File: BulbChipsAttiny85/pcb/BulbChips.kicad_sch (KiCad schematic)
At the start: 27 parts, among them J1 USB_C_Receptacle_USB2.0_14P, J2 LED_2pin_Socket, SW1 SW_Push, U1 DMN52D0UV, U2 USBLC6-2P6, U3 S-82A1ACA-I6T1U, U4 ATtiny85-20M, U5 BQ24045DSQR

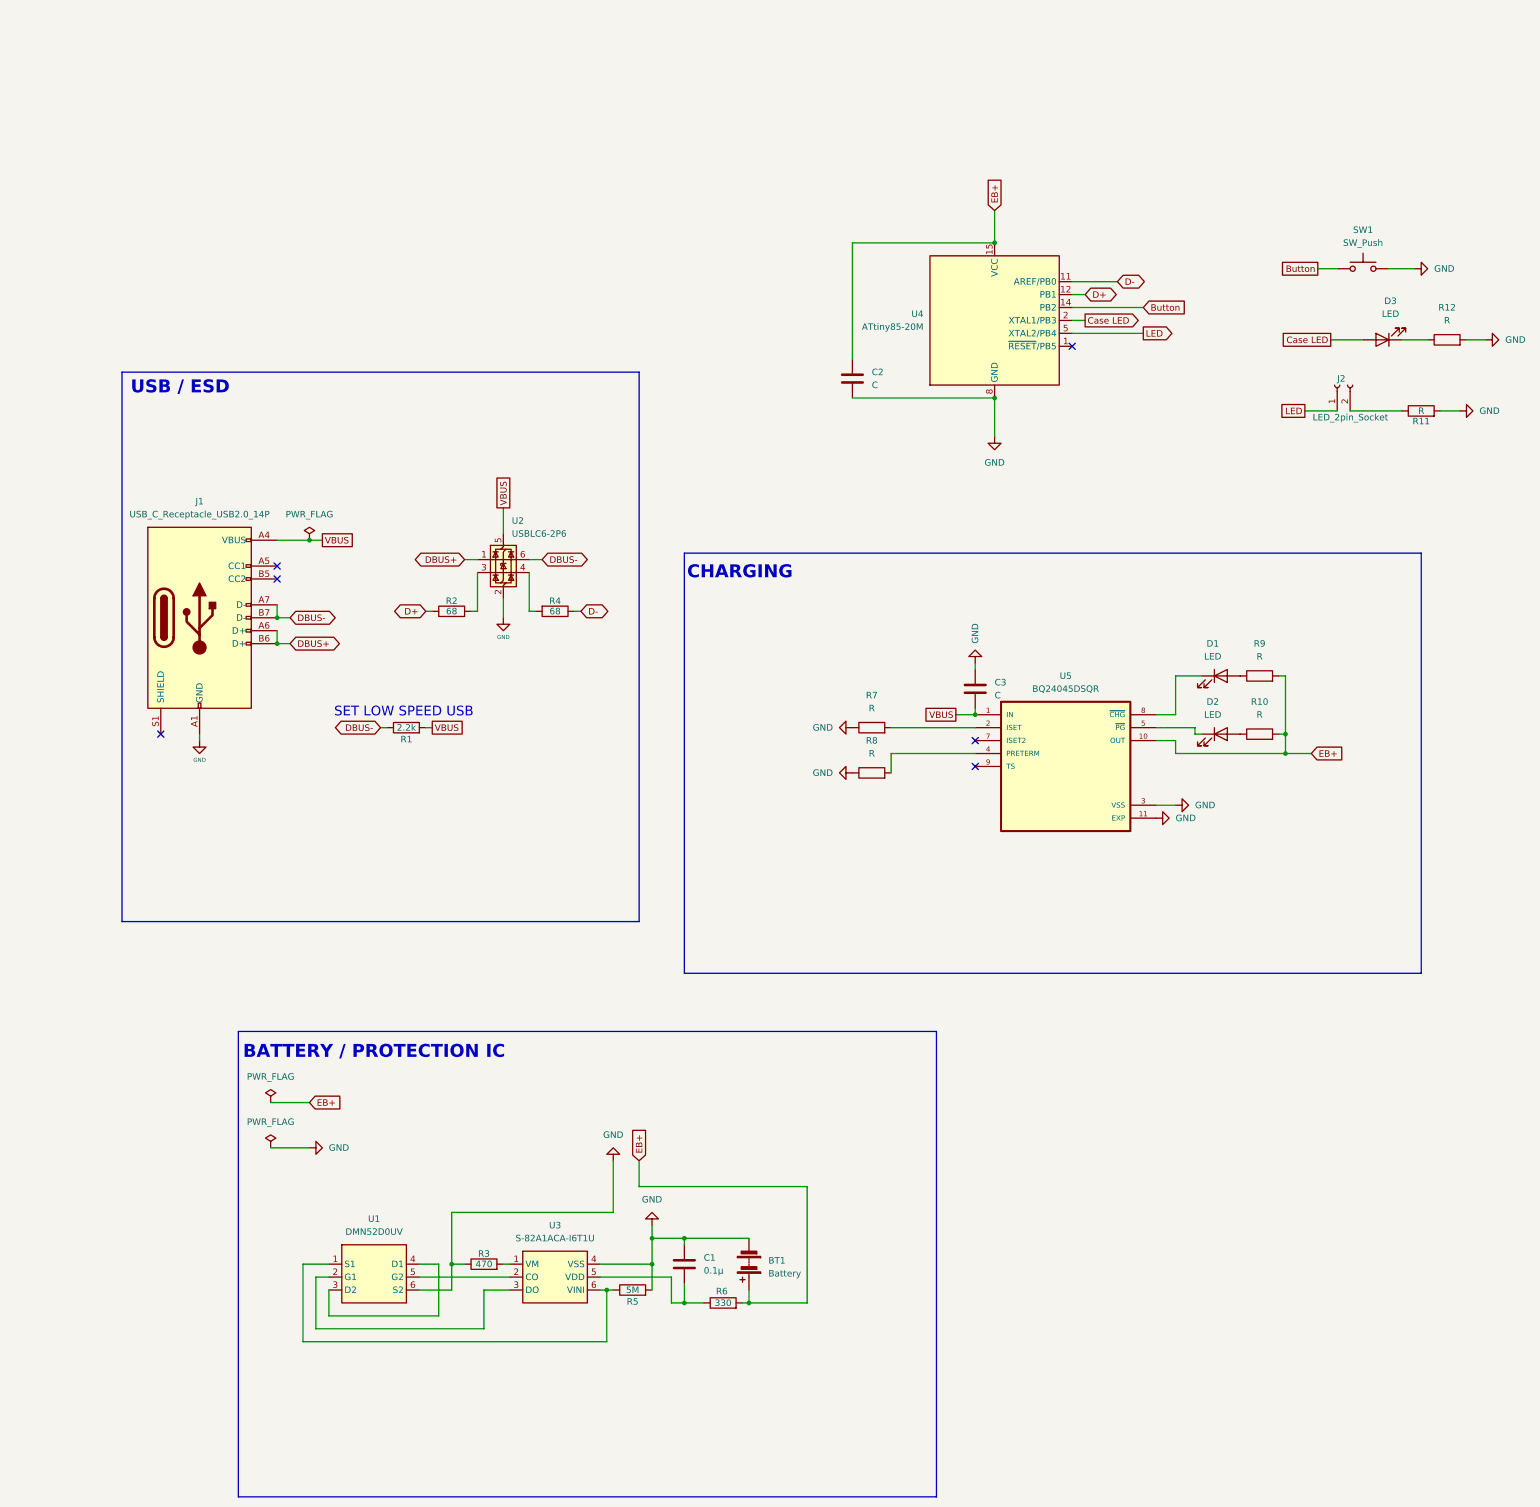
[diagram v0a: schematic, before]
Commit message: organization and labeling
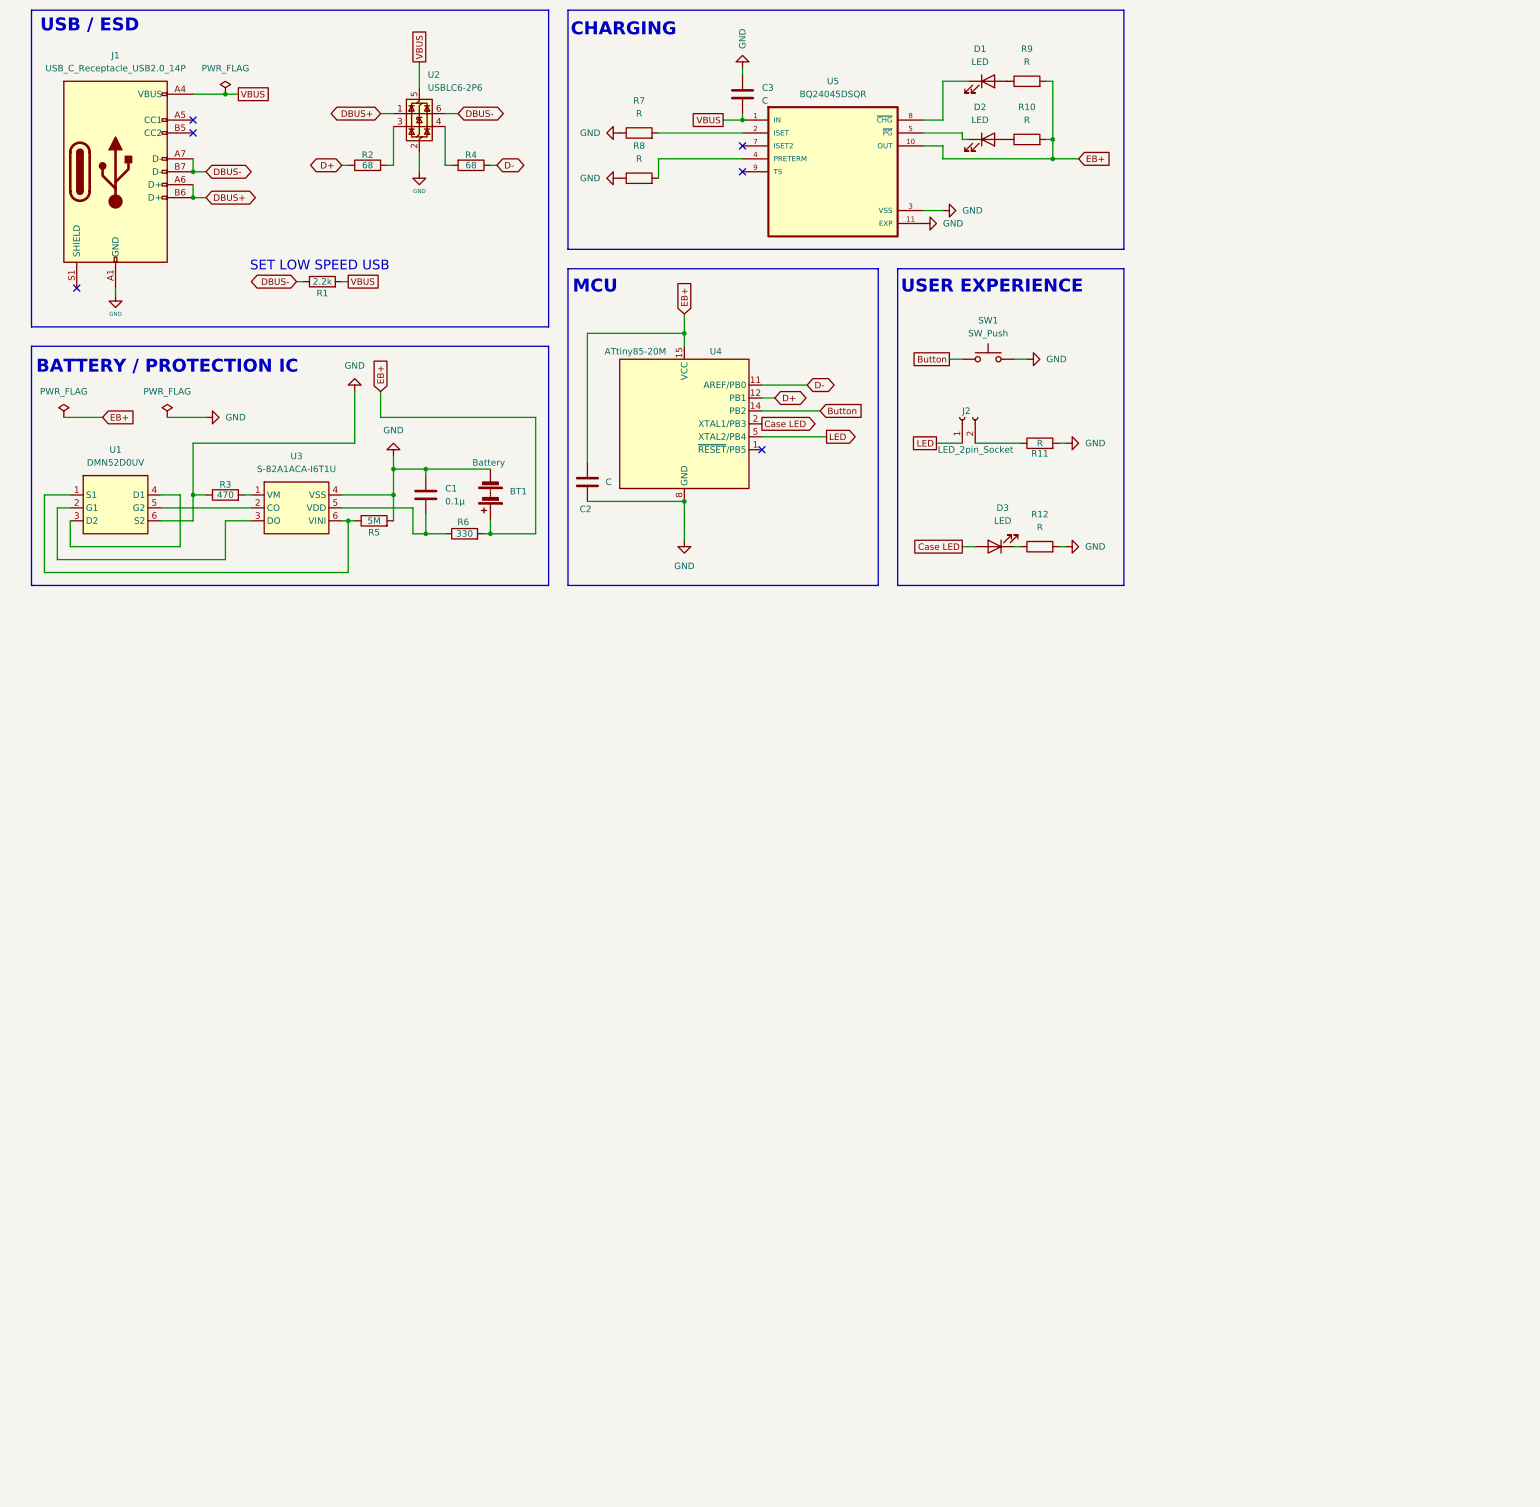
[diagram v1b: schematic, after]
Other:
- note added: "MCU"
- note added: "USER EXPERIENCE"
- moved on the sheet: BT1, C1, C2, C3, D1, D2, D3, J1, J2, R1, R10, R11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
